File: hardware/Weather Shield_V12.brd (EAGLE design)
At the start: 53.3 x 59.7 mm, 52 parts, among them J1 GP-735, Q1 200mA/50V, Q2 200mA/50V, U1 ARDUINO_R3_SHIELD, U3 ALS-PT19, U4 MPL3115A2LGA8, U5 SI7021, U6 3.3V/150mA

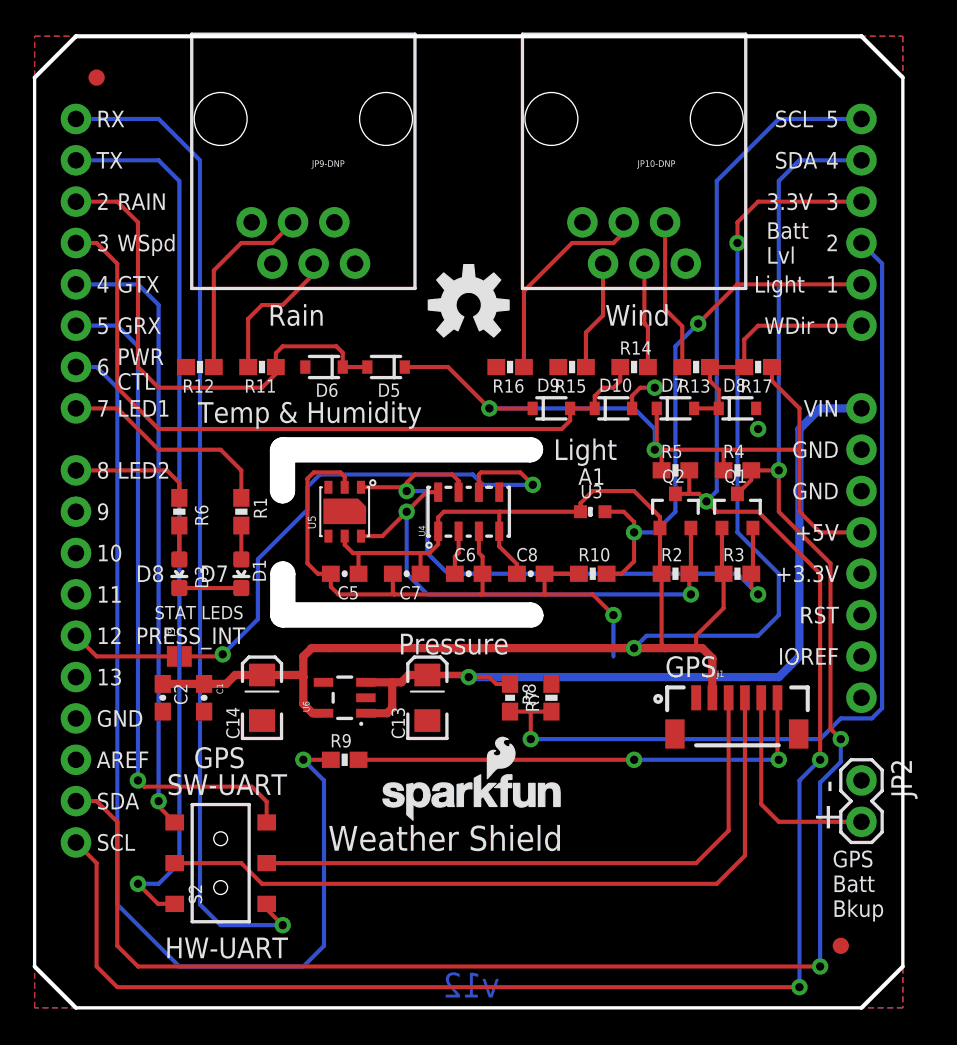
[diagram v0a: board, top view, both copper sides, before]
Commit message: Final issue fixes before going out for reds.
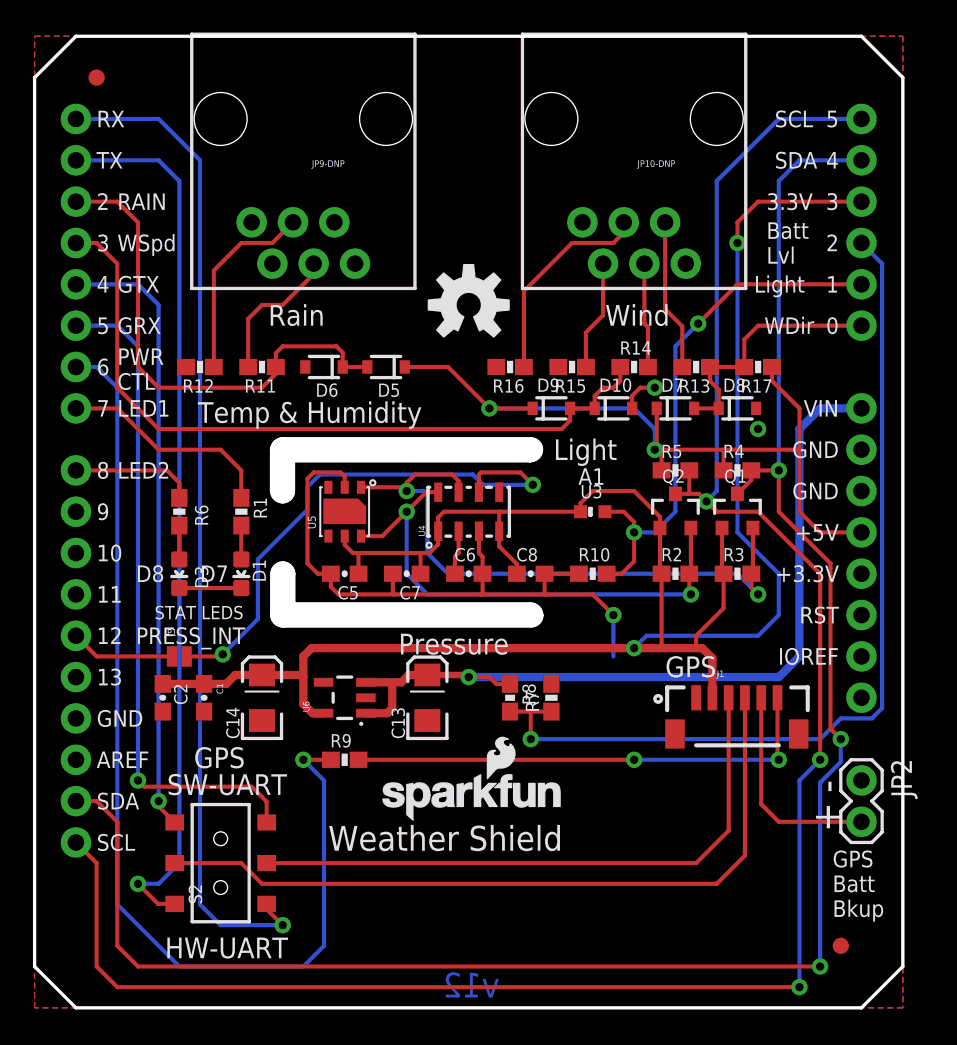
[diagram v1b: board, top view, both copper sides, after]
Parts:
- D10, D5, D6, D7, D8, D9: value (none) -> 250mA/100V
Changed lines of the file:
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@@
 <text x="38.735" y="20.32" size="1.27" layer="21" font="vector" ratio="15">GPS</text>
 <wire x1="2.54" y1="0" x2="50.8" y2="0" width="0.2032" layer="20"/>
-<wire x1="0" y1="57.15" x2="2.54" y2="59.69" width="0.254" layer="20"/>
-<wire x1="2.54" y1="59.69" x2="50.8" y2="59.69" width="0.254" layer="20"/>
-<wire x1="50.8" y1="59.69" x2="53.34" y2="57.15" width="0.254" layer="20"/>
-<wire x1="53.34" y1="2.54" x2="50.8" y2="0" width="0.254" layer="20"/>
-<wire x1="2.54" y1="0" x2="0" y2="2.54" width="0.254" layer="20"/>
+<wire x1="0" y1="57.15" x2="2.54" y2="59.69" width="0.2032" layer="20"/>
+<wire x1="2.54" y1="59.69" x2="50.8" y2="59.69" width="0.2032" layer="20"/>
+<wire x1="50.8" y1="59.69" x2="53.34" y2="57.15" width="0.2032" layer="20"/>
+<wire x1="53.34" y1="2.54" x2="50.8" y2="0" width="0.2032" layer="20"/>
+<wire x1="2.54" y1="0" x2="0" y2="2.54" width="0.2032" layer="20"/>
 <text x="14.351" y="41.91" size="1.27" layer="21" font="vector" ratio="15">Rain</text>
 <text x="35.052" y="41.91" size="1.27" layer="21" font="vector" ratio="15">Wind</text>
@@
 <attribute name="PROD_ID" value="RES-07856" x="40.64" y="39.37" size="1.778" layer="27" rot="R180" display="off"/>
 </element>
-<element name="D9" library="SparkFun-DiscreteSemi" package="SOD-323" value="" x="31.75" y="36.83" smashed="yes">
+<element name="D9" library="SparkFun-DiscreteSemi" package="SOD-323" value="250mA/100V" x="31.75" y="36.83" smashed="yes">
 <attribute name="NAME" x="30.861" y="37.846" size="0.8128" layer="25"/>
 <attribute name="VALUE" value="250mA/100V" x="30.734" y="35.433" size="0.8128" layer="27"/>
 <attribute name="PROD_ID" value="DIO-09646" x="31.75" y="36.83" size="1.778" layer="27" display="off"/>
 </element>
-<element name="D10" library="SparkFun-DiscreteSemi" package="SOD-323" value="" x="35.56" y="36.83" smashed="yes">
+<element name="D10" library="SparkFun-DiscreteSemi" package="SOD-323" value="250mA/100V" x="35.56" y="36.83" smashed="yes">
 <attribute name="NAME" x="34.671" y="37.846" size="0.8128" layer="25"/>
 <attribute name="VALUE" value="250mA/100V" x="34.544" y="35.433" size="0.8128" layer="27"/>
 <attribute name="PROD_ID" value="DIO-09646" x="35.56" y="36.83" size="1.778" layer="27" display="off"/>
 </element>
-<element name="D7" library="SparkFun-DiscreteSemi" package="SOD-323" value="" x="39.37" y="36.83" smashed="yes">
+<element name="D7" library="SparkFun-DiscreteSemi" package="SOD-323" value="250mA/100V" x="39.37" y="36.83" smashed="yes">
 <attribute name="NAME" x="38.481" y="37.846" size="0.8128" layer="25"/>
 <attribute name="VALUE" value="250mA/100V" x="38.354" y="35.433" size="0.8128" layer="27"/>
 <attribute name="PROD_ID" value="DIO-09646" x="39.37" y="36.83" size="1.778" layer="27" display="off"/>
 </element>
-<element name="D8" library="SparkFun-DiscreteSemi" package="SOD-323" value="" x="43.18" y="36.83" smashed="yes">
+<element name="D8" library="SparkFun-DiscreteSemi" package="SOD-323" value="250mA/100V" x="43.18" y="36.83" smashed="yes">
 <attribute name="NAME" x="42.291" y="37.846" size="0.8128" layer="25"/>
 <attribute name="VALUE" value="250mA/100V" x="42.164" y="35.433" size="0.8128" layer="27"/>
 <attribute name="PROD_ID" value="DIO-09646" x="43.18" y="36.83" size="1.778" layer="27" display="off"/>
 </element>
-<element name="D5" library="SparkFun-DiscreteSemi" package="SOD-323" value="" x="21.59" y="39.37" smashed="yes" rot="R180">
+<element name="D5" library="SparkFun-DiscreteSemi" package="SOD-323" value="250mA/100V" x="21.59" y="39.37" smashed="yes" rot="R180">
 <attribute name="NAME" x="22.479" y="38.354" size="0.8128" layer="25" rot="R180"/>
 <attribute name="VALUE" value="250mA/100V" x="22.606" y="40.767" size="0.8128" layer="27" rot="R180"/>
 <attribute name="PROD_ID" value="DIO-09646" x="21.59" y="39.37" size="1.778" layer="27" rot="R180" display="off"/>
 </element>
-<element name="D6" library="SparkFun-DiscreteSemi" package="SOD-323" value="" x="17.78" y="39.37" smashed="yes" rot="R180">
+<element name="D6" library="SparkFun-DiscreteSemi" package="SOD-323" value="250mA/100V" x="17.78" y="39.37" smashed="yes" rot="R180">
 <attribute name="NAME" x="18.669" y="38.354" size="0.8128" layer="25" rot="R180"/>
 <attribute name="VALUE" value="250mA/100V" x="18.796" y="40.767" size="0.8128" layer="27" rot="R180"/>
